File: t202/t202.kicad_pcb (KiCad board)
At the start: 2 copper layers, 24.2 x 12.2 mm, 12 parts, among them J1 Conn_02x04_Counter_Clockwise, SW1 SW_Push, SW2 SW_SPDT, U1 ATtiny202-SS, U3 CH340K

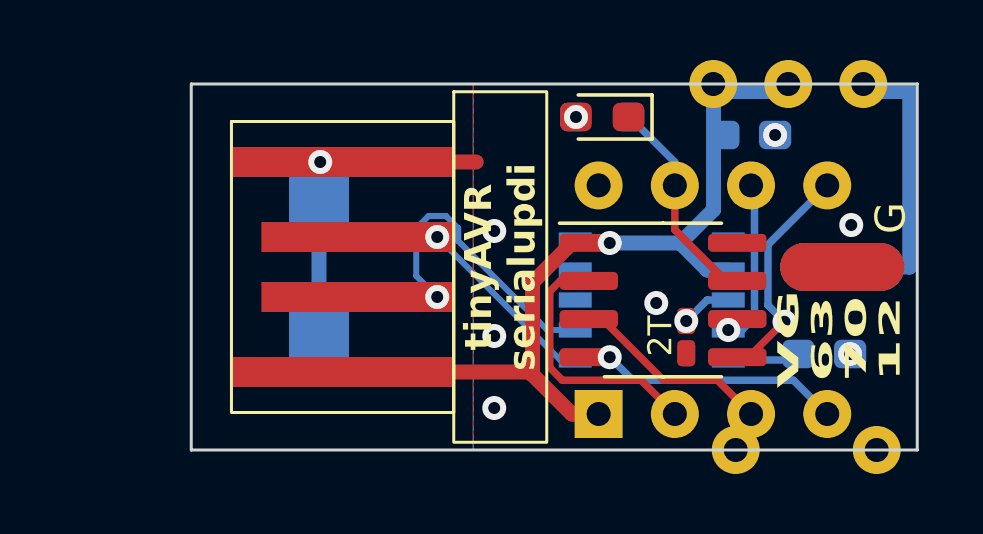
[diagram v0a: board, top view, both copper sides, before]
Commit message: -
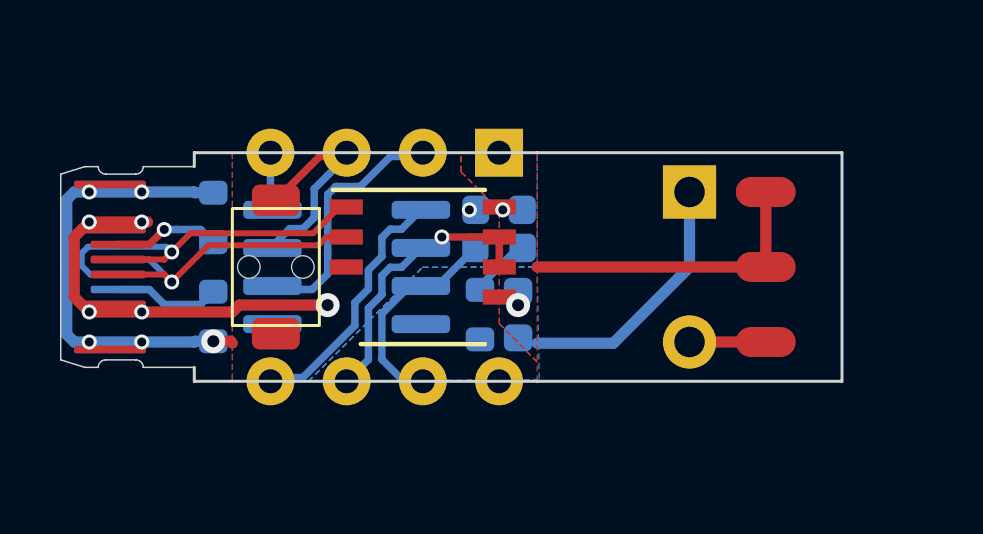
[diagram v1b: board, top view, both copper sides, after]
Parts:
- removed JP1: SolderJumper_2_Open, Library:sop_jumper
- removed U3: CH340K, Package_SO:SSOP-10_3.9x4.9mm_P1.00mm
- added R5: 5k1, Resistor_SMD:R_0603_1608Metric, B.Cu at (100.6, 98.3)
- added R6: 5k1, Resistor_SMD:R_0603_1608Metric, B.Cu at (100.6, 101.7)
- added U2: CH340K, Package_SO:SSOP-10_3.9x4.9mm_P1.00mm, F.Cu at (107.6, 100.0)
- C1: value 0u1 -> 4u7; footprint Capacitor_SMD:C_0603_1608Metric_Pad1.08x0.95mm_HandSolder -> Capacitor_SMD:C_0603_1608Metric
- C2: value 0u1 -> 1F5; footprint Capacitor_SMD:C_0603_1608Metric_Pad1.08x0.95mm_HandSolder -> Library:edlc; moved to F.Cu
- C3: value 1.5F -> 0u1; footprint Library:ELDC_v -> Capacitor_SMD:C_0603_1608Metric
- D1: footprint LED_SMD:LED_0603_1608Metric_Pad1.05x0.95mm_HandSolder -> LED_SMD:LED_0603_1608Metric; moved to B.Cu
- J1: value Conn_02x04_Counter_Clockwise -> USB-C; footprint Package_DIP:DIP-8_W7.62mm -> Library:USB-C
- J2: value ~ -> OUT; footprint Library:PCB_USB_Conn -> Package_DIP:DIP-8_W7.62mm_Socket
- R1: footprint Resistor_SMD:R_0603_1608Metric_Pad0.98x0.95mm_HandSolder -> Resistor_SMD:R_0603_1608Metric
- SW1: footprint Library:TVAF06-A020B-R -> Library:sw_push_smd
- SW2: footprint Library:3pad_2.5_h -> Library:sw
- U1: moved to B.Cu
- moved SW1 18.7 mm to (102.7, 100.0), turned to -90 degrees
- moved J1 14.3 mm to (100.0, 100.0), turned to 180 degrees
- moved C3 13.6 mm to (110.2, 98.1), turned to 180 degrees
- moved J2 10.9 mm to (110.2, 96.2), turned to -90 degrees
- moved U1 10.6 mm to (105.1, 100.0)
- moved C1 9.76 mm to (110.8, 101.6), turned to -90 degrees
- moved R1 7.75 mm to (109.5, 101.6), turned to -90 degrees
- moved SW2 6.15 mm to (119.0, 100.0), turned to 0 degrees
- moved D1 5.56 mm to (110.2, 99.4)
- moved C2 5.35 mm to (116.5, 100.0), turned to 180 degrees
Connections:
- C1 pad 1: +5V -> VCC
- C2 pad 1: Net-(U3-V3) -> /Vedlc
- C3 pad 1: Net-(SW2-C) -> Net-(U2-V3)
- D1 pad 1: GND -> Net-(D1-K)
- D1 pad 2: Net-(D1-A) -> PA3
- J1 pad 1: +5V -> GND
- J1 pad 2: PA6 -> D+
- J1 pad 3: PA7 -> D-
- J1 pad 4: PA1 -> VCC
- J1 pad 5: PA2 -> Net-(J1-CC1)
- J1 pad 6: PA0 -> Net-(J1-CC2)
- J2 pad 1: GND -> VCC
- J2 pad 2: D+ -> PA6
- J2 pad 3: D- -> PA7
- J2 pad 4: +5V -> PA1
- J2 pad 5: GND -> PA2
- J2 pad 6: GND -> UPDI
- R1 pad 1: PA3 -> Net-(D1-K)
- R1 pad 2: Net-(D1-A) -> GND
- SW1 pad 1: PA7 -> GND
- SW1 pad 2: GND -> PA7
- SW2 pad 1: +5V -> VCC
- SW2 pad 2: +5V -> VCC
- SW2 pad 3: Net-(SW2-C) -> /Vedlc
- U1 pad 1: +5V -> VCC
- U1 pad 6: PA0 -> UPDI
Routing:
- net +5V: track 27.6 -> 0.00 mm, vias 1 -> 0
- net VCC: track 0.00 -> 23.5 mm, vias 0 -> 6
- net GND: track 9.96 -> 23.8 mm, vias 8 -> 6
- net Net-(SW2-C): track 9.65 -> 0.00 mm
- net UPDI: track 0.00 -> 9.41 mm, vias 0 -> 1
- net PA1: track 8.73 -> 1.81 mm, vias 1 -> 0
- net PA0: track 5.50 -> 0.00 mm, vias 1 -> 0
- net D+: track 8.95 -> 13.2 mm
- net Net-(J1-CC2): track 0.00 -> 3.55 mm
- net Net-(J1-CC1): track 0.00 -> 3.55 mm, vias 0 -> 1
- net /Vedlc: track 0.00 -> 2.54 mm
- net Net-(U3-V3): track 2.42 -> 0.00 mm
- net D-: track 12.5 -> 10.4 mm
- net Net-(D1-K): track 0.00 -> 2.08 mm
- net Net-(JP1-B): track 1.69 -> 0.00 mm, vias 1 -> 0
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- added copper zone on B.Cu, net VCC
- added copper zone on F.Cu, net VCC
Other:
- board size 24.2 x 12.2 mm -> 21.6 x 7.6 mm
- board text added: "ATtiny202 USB-C"
- board text removed: "2T"
- board text removed: "G"
- board text removed: "TR"
- board text removed: "VG 63 70 12"
- board text removed: "Vbat"
- board text removed: "tinyAVR serialupdi"
